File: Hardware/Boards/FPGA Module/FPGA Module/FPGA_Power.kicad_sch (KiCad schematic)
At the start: 1 part, among them U1 XCKU3P-FFVA676

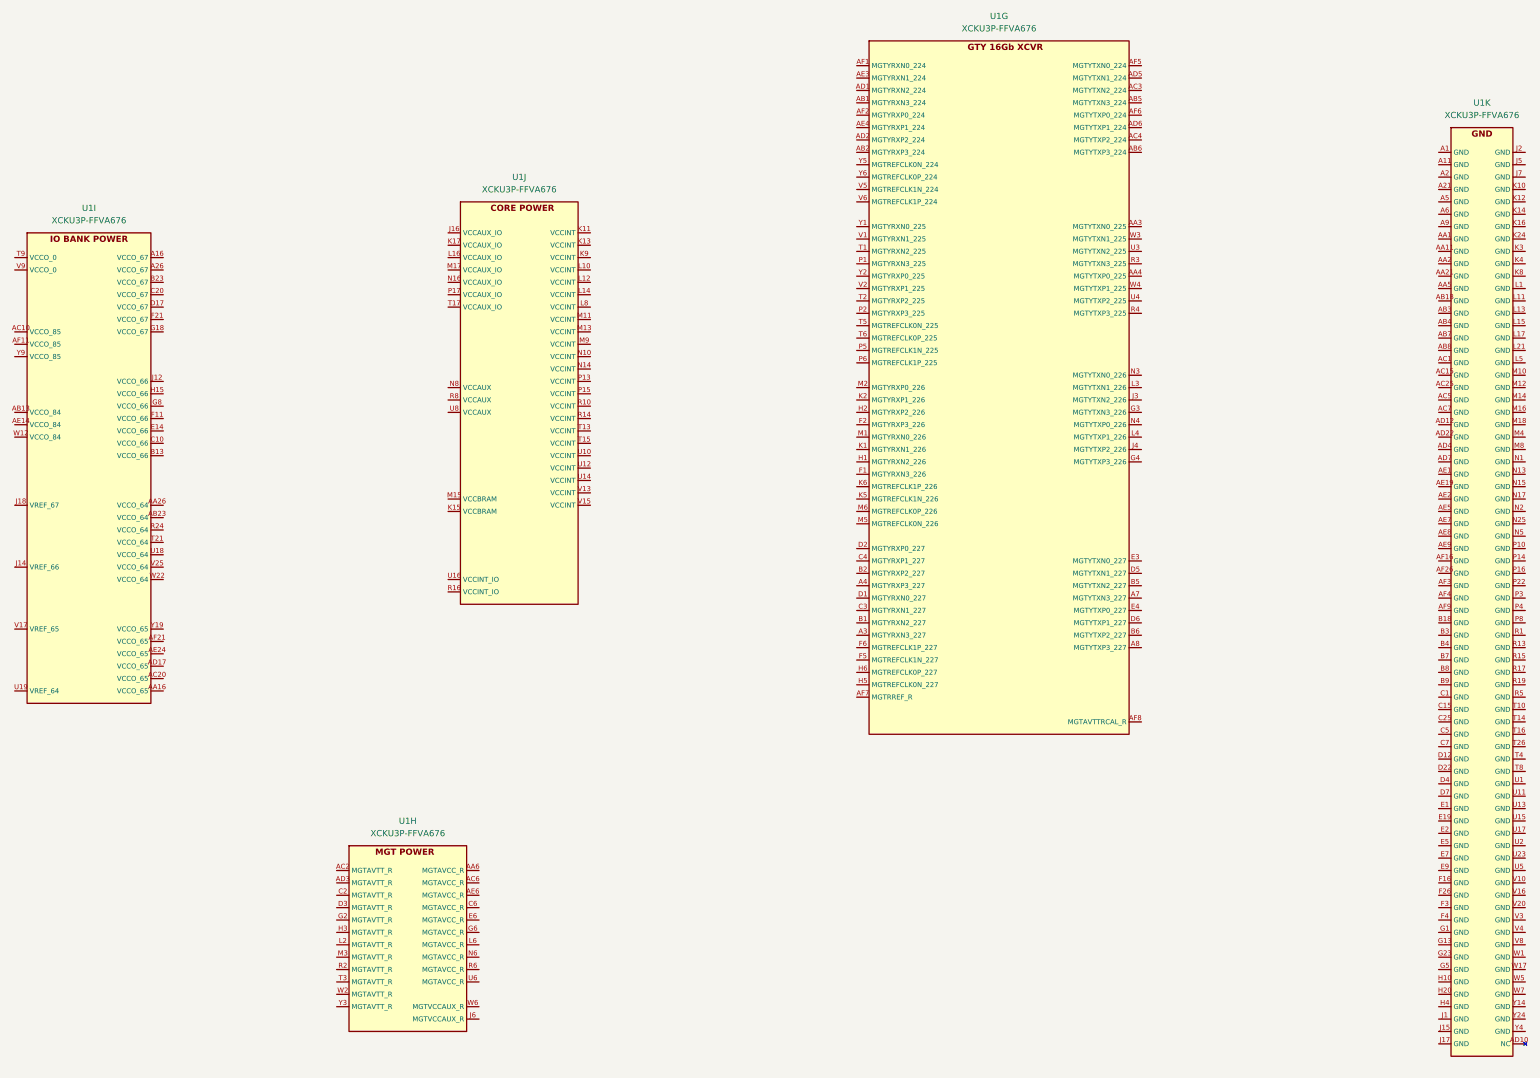
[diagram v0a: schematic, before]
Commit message: Added FPGA Config page
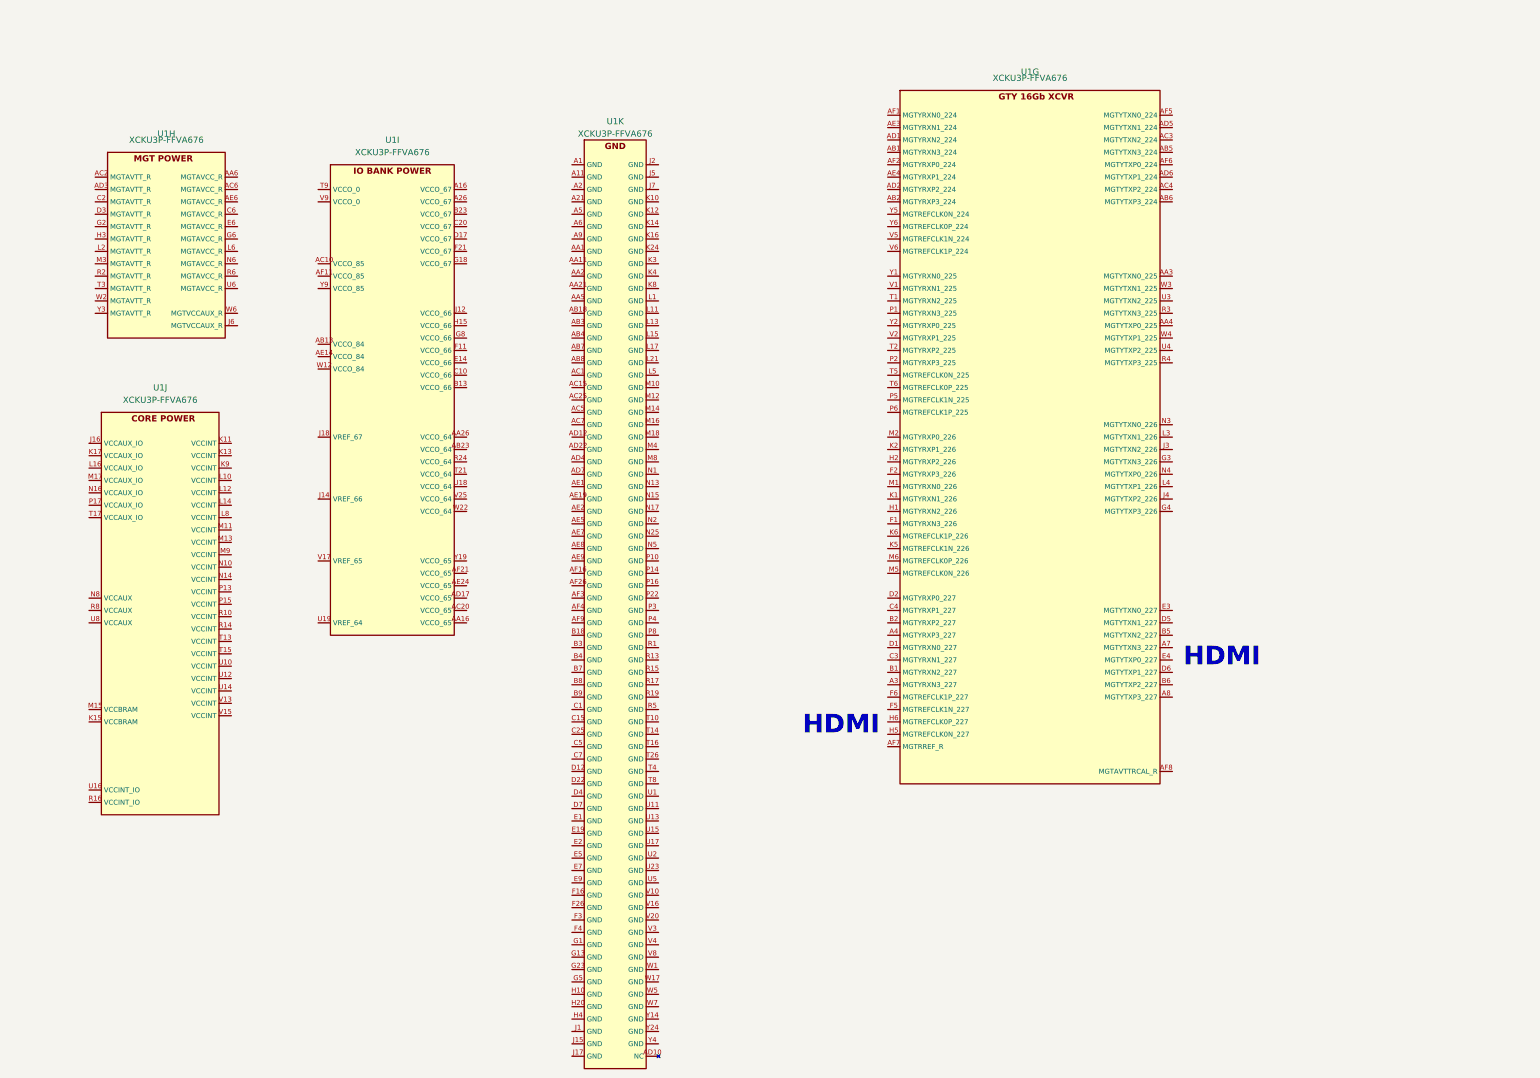
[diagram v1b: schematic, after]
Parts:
- removed U1: XCKU3P-FFVA676, DICE_FPGA_Module:BGA676, symbol DICE_FPGA_Module:XCKU3P-FFVA676
- added U1: XCKU3P-FFVA676, FPGA Module:BGA676, symbol FPGA Module:XCKU3P-FFVA676
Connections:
- new net: U1.AD10 (NC), U1.AE13 (NC), U1.E24 (NC), U1.E25 (NC), U1.E26 (NC), U1.F22 (NC), U1.F23 (NC), U1.F24 (NC), U1.F25 (NC), U1.G20 (NC), U1.G21 (NC), U1.G22 (NC), U1.G24 (NC), U1.G25 (NC), U1.G26 (NC), U1.H19 (NC), U1.H21 (NC), U1.H22 (NC), U1.H23 (NC), U1.H24 (NC), U1.H25 (NC), U1.H26 (NC), U1.J19 (NC), U1.J20 (NC), U1.J21 (NC), U1.J22 (NC), U1.J23 (NC), U1.J24 (NC), U1.J25 (NC), U1.J26 (NC), U1.K18 (NC), U1.K19 (NC), U1.K20 (NC), U1.K21 (NC), U1.K22 (NC), U1.K23 (NC), U1.K25 (NC), U1.K26 (NC), U1.L18 (NC), U1.L19 (NC), U1.L20 (NC), U1.L22 (NC), U1.L23 (NC), U1.L24 (NC), U1.L25 (NC), U1.L26 (NC), U1.M19 (NC), U1.M20 (NC), U1.M21 (NC), U1.M22 (NC), U1.M23 (NC), U1.M24 (NC), U1.M25 (NC), U1.M26 (NC), U1.N18 (NC), U1.N19 (NC), U1.N20 (NC), U1.N21 (NC), U1.N22 (NC), U1.N23 (NC), U1.N24 (NC), U1.N26 (NC), U1.V14 (NC), U1.Y12 (NC), U1.Y13 (NC)
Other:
- note added: "HDMI"
